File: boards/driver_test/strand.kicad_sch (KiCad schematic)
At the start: 8 parts, among them Q24 MMBT2222, Q25 MMBT2907

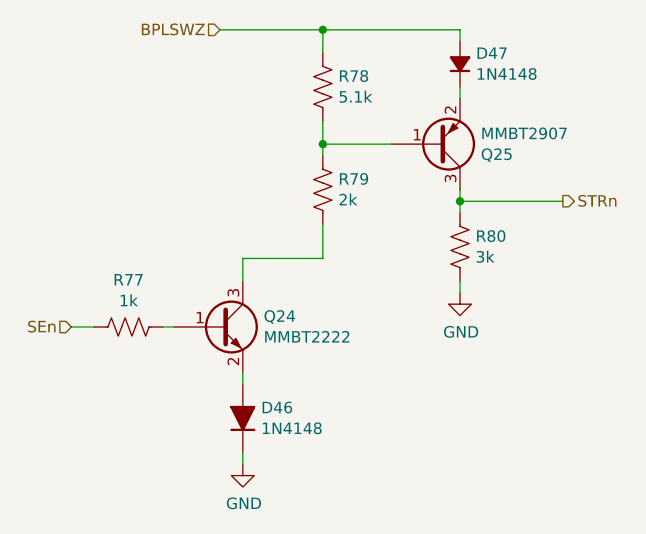
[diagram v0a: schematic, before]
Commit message: Driver test: updated schematic with new coarse tuning resistance values for all 3 current driver types
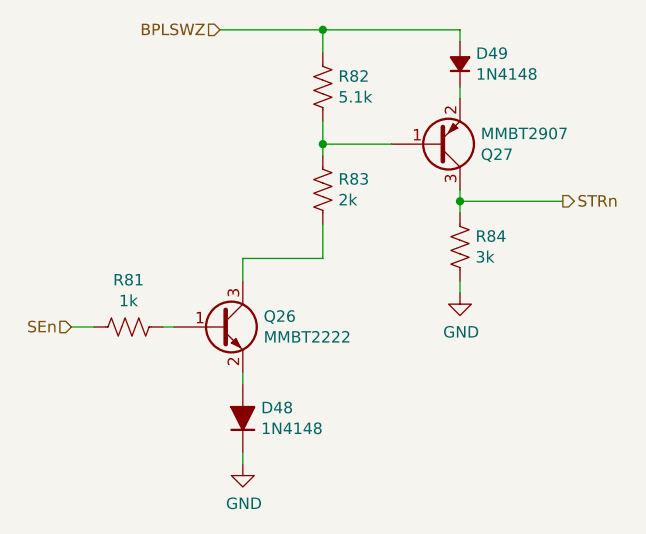
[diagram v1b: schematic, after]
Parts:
- renumbered D46 to D48, D47 to D49, Q24 to Q26, Q25 to Q27, R77 to R81, R78 to R82, R79 to R83, R80 to R84
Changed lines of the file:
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@@
   (symbol (lib_id "power:GND") (at 157.48 99.06 0)
     (in_bom yes) (on_board yes)
-    (property "Reference" "#PWR068" (id 0) (at 157.48 105.41 0)
+    (property "Reference" "#PWR070" (id 0) (at 157.48 105.41 0)
       (effects (font (size 1.27 1.27)) hide)
     )
@@
   (symbol (lib_id "Device:R_US") (at 142.24 87.63 0)
     (in_bom yes) (on_board yes)
-    (property "Reference" "R79" (id 0) (at 143.9672 86.4616 0)
+    (property "Reference" "R83" (id 0) (at 143.9672 86.4616 0)
       (effects (font (size 1.27 1.27)) (justify left))
     )
@@
   (symbol (lib_id "Device:R_US") (at 142.24 76.2 0)
     (in_bom yes) (on_board yes)
-    (property "Reference" "R78" (id 0) (at 143.9672 75.0316 0)
+    (property "Reference" "R82" (id 0) (at 143.9672 75.0316 0)
       (effects (font (size 1.27 1.27)) (justify left))
     )
@@
   (symbol (lib_id "Device:Q_PNP_BEC") (at 154.94 82.55 0) (mirror x)
     (in_bom yes) (on_board yes)
-    (property "Reference" "Q25" (id 0) (at 159.7914 83.7184 0)
+    (property "Reference" "Q27" (id 0) (at 159.7914 83.7184 0)
       (effects (font (size 1.27 1.27)) (justify left))
     )
@@
   (symbol (lib_id "Device:R_US") (at 157.48 93.98 0)
     (in_bom yes) (on_board yes)
-    (property "Reference" "R80" (id 0) (at 159.2072 92.8116 0)
+    (property "Reference" "R84" (id 0) (at 159.2072 92.8116 0)
       (effects (font (size 1.27 1.27)) (justify left))
     )
@@
   (symbol (lib_id "Device:D_Small_Filled") (at 157.48 73.66 90)
     (in_bom yes) (on_board yes)
-    (property "Reference" "D47" (id 0) (at 159.258 72.4916 90)
+    (property "Reference" "D49" (id 0) (at 159.258 72.4916 90)
       (effects (font (size 1.27 1.27)) (justify right))
     )
@@
   (symbol (lib_id "Device:R_US") (at 120.65 102.87 270)
     (in_bom yes) (on_board yes)
-    (property "Reference" "R77" (id 0) (at 120.65 97.663 90))
+    (property "Reference" "R81" (id 0) (at 120.65 97.663 90))
     (property "Value" "1k" (id 1) (at 120.65 99.9744 90))
     (property "Footprint" "Resistor_SMD:R_0603_1608Metric" (id 2) (at 120.396 103.886 90)
@@
   (symbol (lib_id "Device:Q_NPN_BEC") (at 130.81 102.87 0)
     (in_bom yes) (on_board yes)
-    (property "Reference" "Q24" (id 0) (at 135.6614 101.7016 0)
+    (property "Reference" "Q26" (id 0) (at 135.6614 101.7016 0)
       (effects (font (size 1.27 1.27)) (justify left))
     )
@@
   (symbol (lib_id "Device:D_Filled") (at 133.35 113.03 90)
     (in_bom yes) (on_board yes)
-    (property "Reference" "D46" (id 0) (at 135.382 111.8616 90)
+    (property "Reference" "D48" (id 0) (at 135.382 111.8616 90)
       (effects (font (size 1.27 1.27)) (justify right))
     )
@@
   (symbol (lib_id "power:GND") (at 133.35 118.11 0)
     (in_bom yes) (on_board yes)
-    (property "Reference" "#PWR067" (id 0) (at 133.35 124.46 0)
+    (property "Reference" "#PWR069" (id 0) (at 133.35 124.46 0)
       (effects (font (size 1.27 1.27)) hide)
     )

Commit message: Driver test: dropped BPLSSW LED brightness by bumping its resistor up to 1k
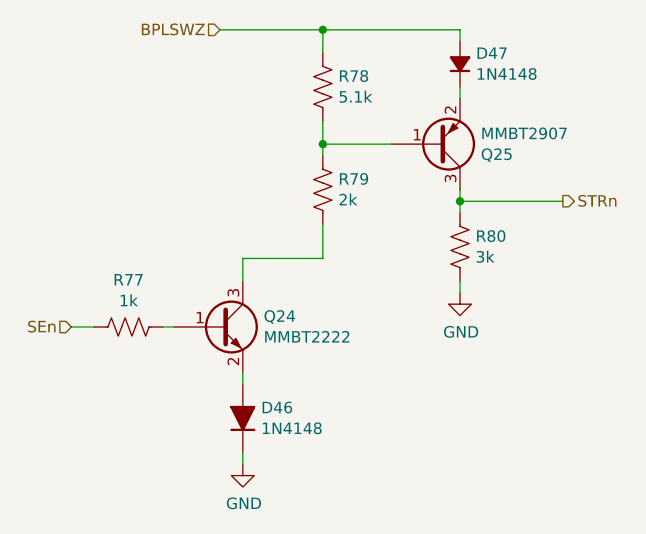
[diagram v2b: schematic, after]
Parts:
- renumbered D48 to D46, D49 to D47, Q26 to Q24, Q27 to Q25, R81 to R77, R82 to R78, R83 to R79, R84 to R80
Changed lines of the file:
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@@
   (symbol (lib_id "power:GND") (at 157.48 99.06 0)
     (in_bom yes) (on_board yes)
-    (property "Reference" "#PWR070" (id 0) (at 157.48 105.41 0)
+    (property "Reference" "#PWR068" (id 0) (at 157.48 105.41 0)
       (effects (font (size 1.27 1.27)) hide)
     )
@@
   (symbol (lib_id "Device:R_US") (at 142.24 87.63 0)
     (in_bom yes) (on_board yes)
-    (property "Reference" "R83" (id 0) (at 143.9672 86.4616 0)
+    (property "Reference" "R79" (id 0) (at 143.9672 86.4616 0)
       (effects (font (size 1.27 1.27)) (justify left))
     )
@@
   (symbol (lib_id "Device:R_US") (at 142.24 76.2 0)
     (in_bom yes) (on_board yes)
-    (property "Reference" "R82" (id 0) (at 143.9672 75.0316 0)
+    (property "Reference" "R78" (id 0) (at 143.9672 75.0316 0)
       (effects (font (size 1.27 1.27)) (justify left))
     )
@@
   (symbol (lib_id "Device:Q_PNP_BEC") (at 154.94 82.55 0) (mirror x)
     (in_bom yes) (on_board yes)
-    (property "Reference" "Q27" (id 0) (at 159.7914 83.7184 0)
+    (property "Reference" "Q25" (id 0) (at 159.7914 83.7184 0)
       (effects (font (size 1.27 1.27)) (justify left))
     )
@@
   (symbol (lib_id "Device:R_US") (at 157.48 93.98 0)
     (in_bom yes) (on_board yes)
-    (property "Reference" "R84" (id 0) (at 159.2072 92.8116 0)
+    (property "Reference" "R80" (id 0) (at 159.2072 92.8116 0)
       (effects (font (size 1.27 1.27)) (justify left))
     )
@@
   (symbol (lib_id "Device:D_Small_Filled") (at 157.48 73.66 90)
     (in_bom yes) (on_board yes)
-    (property "Reference" "D49" (id 0) (at 159.258 72.4916 90)
+    (property "Reference" "D47" (id 0) (at 159.258 72.4916 90)
       (effects (font (size 1.27 1.27)) (justify right))
     )
@@
   (symbol (lib_id "Device:R_US") (at 120.65 102.87 270)
     (in_bom yes) (on_board yes)
-    (property "Reference" "R81" (id 0) (at 120.65 97.663 90))
+    (property "Reference" "R77" (id 0) (at 120.65 97.663 90))
     (property "Value" "1k" (id 1) (at 120.65 99.9744 90))
     (property "Footprint" "Resistor_SMD:R_0603_1608Metric" (id 2) (at 120.396 103.886 90)
@@
   (symbol (lib_id "Device:Q_NPN_BEC") (at 130.81 102.87 0)
     (in_bom yes) (on_board yes)
-    (property "Reference" "Q26" (id 0) (at 135.6614 101.7016 0)
+    (property "Reference" "Q24" (id 0) (at 135.6614 101.7016 0)
       (effects (font (size 1.27 1.27)) (justify left))
     )
@@
   (symbol (lib_id "Device:D_Filled") (at 133.35 113.03 90)
     (in_bom yes) (on_board yes)
-    (property "Reference" "D48" (id 0) (at 135.382 111.8616 90)
+    (property "Reference" "D46" (id 0) (at 135.382 111.8616 90)
       (effects (font (size 1.27 1.27)) (justify right))
     )
@@
   (symbol (lib_id "power:GND") (at 133.35 118.11 0)
     (in_bom yes) (on_board yes)
-    (property "Reference" "#PWR069" (id 0) (at 133.35 124.46 0)
+    (property "Reference" "#PWR067" (id 0) (at 133.35 124.46 0)
       (effects (font (size 1.27 1.27)) hide)
     )
